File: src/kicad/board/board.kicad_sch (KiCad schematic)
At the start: 24 parts, among them J1 USB_C_Receptacle_USB2.0, J2 Conn_01x06, J3 Micro_SD_Card_Det, J4 Conn_01x05_Male, J5 Conn_01x05_Male

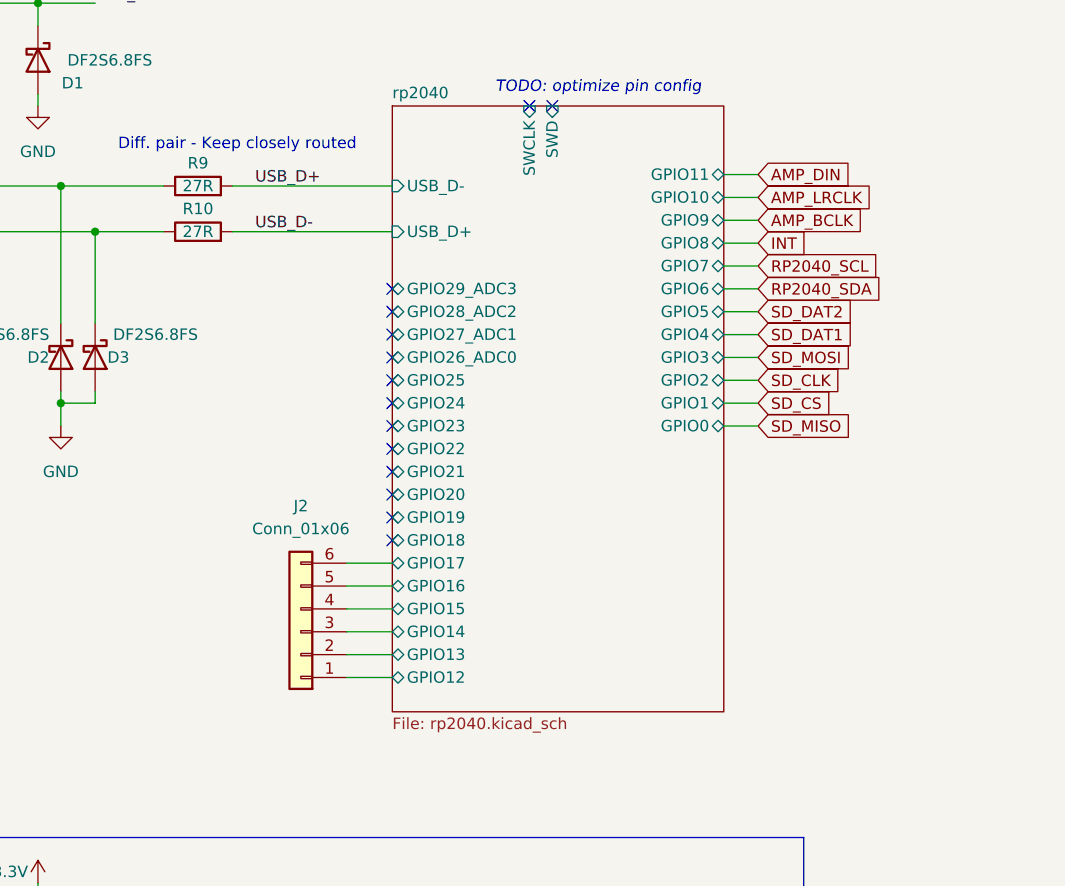
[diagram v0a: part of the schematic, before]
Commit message: update
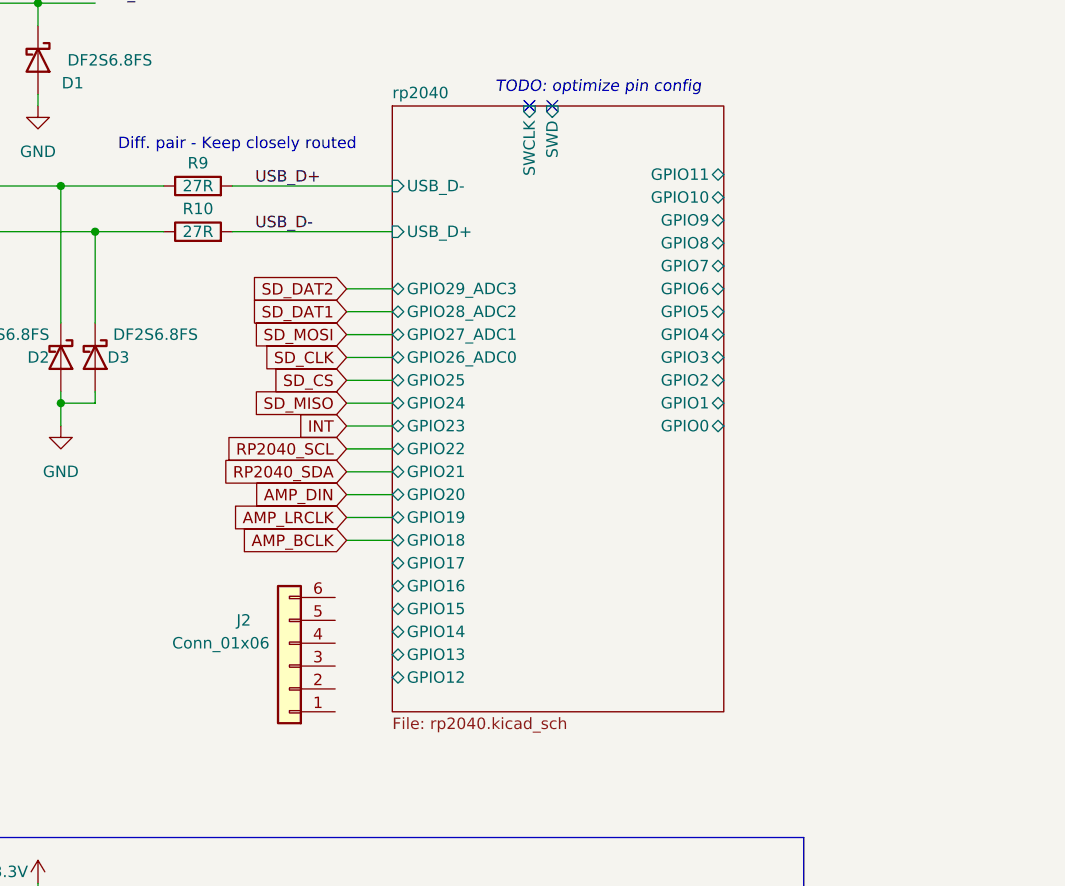
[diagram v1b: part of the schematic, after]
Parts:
- C2: footprint Capacitor_SMD:C_0603_1608Metric -> Capacitor_SMD:C_0402_1005Metric; Vendor C14663 -> C307331
- R10, R9: footprint Resistor_SMD:R_0805_2012Metric -> Resistor_SMD:R_0603_1608Metric; Vendor C17594 -> C25190
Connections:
- net rp2040/GPIO12: no longer J2.1 (Pin_1)
- net rp2040/GPIO13: no longer J2.2 (Pin_2)
- net rp2040/GPIO14: no longer J2.3 (Pin_3)
- net rp2040/GPIO15: no longer J2.4 (Pin_4)
- net rp2040/GPIO16: no longer J2.5 (Pin_5)
- net rp2040/GPIO17: no longer J2.6 (Pin_6)
- no-connect marks 18 -> 6
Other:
- moved on the sheet: J2
